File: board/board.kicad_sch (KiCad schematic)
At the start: 2 parts, among them J1 011_GPIO

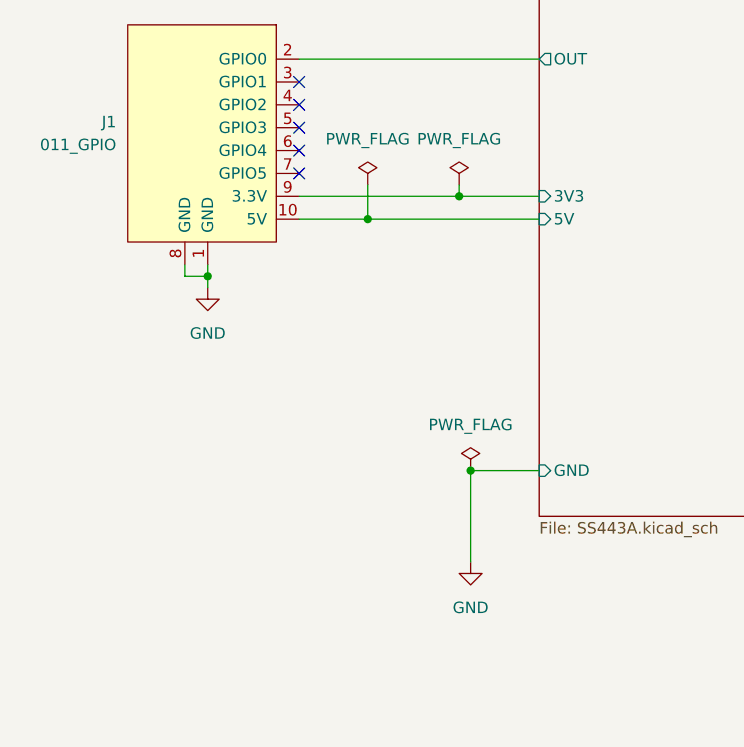
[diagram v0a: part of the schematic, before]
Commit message: Update libraries
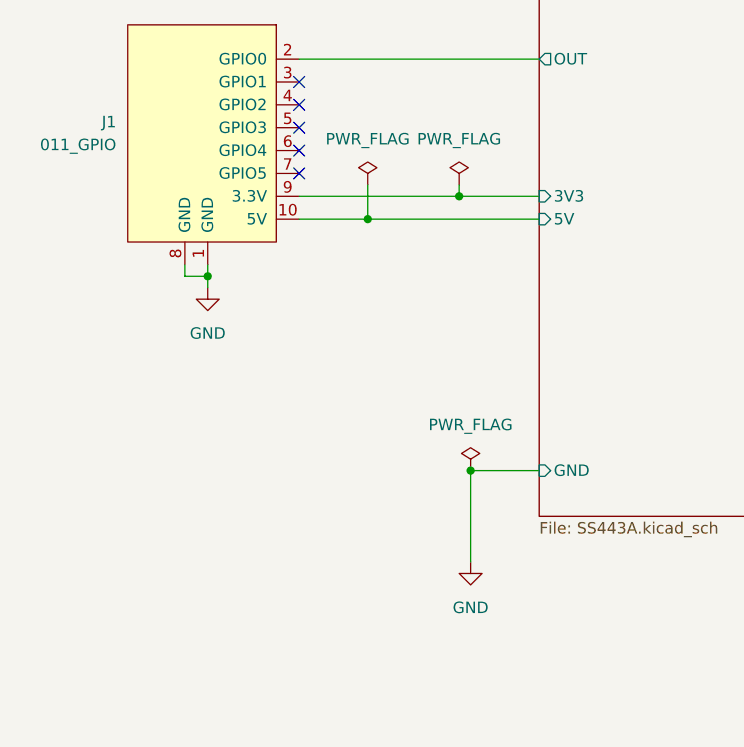
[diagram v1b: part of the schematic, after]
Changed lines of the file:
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@@
   (junction (at 124.46 90.17) (diameter 0) (color 0 0 0 0)
   )
+  (junction (at 96.52 99.06) (diameter 0) (color 0 0 0 0)
+  )
   (junction (at 125.73 120.65) (diameter 0) (color 0 0 0 0)
-  )
-  (junction (at 96.52 99.06) (diameter 0) (color 0 0 0 0)
   )
   (junction (at 114.3 92.71) (diameter 0) (color 0 0 0 0)
@@
     (stroke (width 0) (type default) (color 0 0 0 0))
   )
-  (symbol (lib_id "power:PWR_FLAG") (at 124.46 88.9 0) (mirror y) (unit 1)
-    (in_bom yes) (on_board yes) (fields_autoplaced)
-    (property "Reference" "#FLG0102" (id 0) (at 124.46 86.995 0)
+  (symbol (lib_id "power:PWR_FLAG") (at 124.46 88.9 0) (unit 1)
+    (in_bom yes) (on_board yes) (fields_autoplaced)
+    (property "Reference" "#FLG0103" (id 0) (at 124.46 86.995 0)
       (effects (font (size 1.27 1.27)) hide)
     )
@@
     (pin "1")
   )
-  (symbol (lib_id "power:PWR_FLAG") (at 125.73 120.65 0) (mirror y) (unit 1)
-    (in_bom yes) (on_board yes) (fields_autoplaced)
-    (property "Reference" "#FLG0103" (id 0) (at 125.73 118.745 0)
-      (effects (font (size 1.27 1.27)) hide)
-    )
-    (property "Value" "PWR_FLAG" (id 1) (at 125.73 115.57 0))
-    (property "Footprint" "" (id 2) (at 125.73 120.65 0)
-      (effects (font (size 1.27 1.27)) hide)
-    )
-    (property "Datasheet" "~" (id 3) (at 125.73 120.65 0)
-      (effects (font (size 1.27 1.27)) hide)
-    )
-    (pin "1")
-  )
-  (symbol (lib_id "power:GND") (at 96.52 100.33 0) (mirror y) (unit 1)
-    (in_bom yes) (on_board yes) (fields_autoplaced)
-    (property "Reference" "#PWR0101" (id 0) (at 96.52 106.68 0)
-      (effects (font (size 1.27 1.27)) hide)
-    )
-    (property "Value" "GND" (id 1) (at 96.52 105.41 0))
-    (property "Footprint" "" (id 2) (at 96.52 100.33 0)
-      (effects (font (size 1.27 1.27)) hide)
-    )
-    (property "Datasheet" "" (id 3) (at 96.52 100.33 0)
-      (effects (font (size 1.27 1.27)) hide)
-    )
-    (pin "1")
-  )
-  (symbol (lib_id "power:GND") (at 125.73 130.81 0) (mirror y) (unit 1)
-    (in_bom yes) (on_board yes) (fields_autoplaced)
-    (property "Reference" "#PWR0102" (id 0) (at 125.73 137.16 0)
-      (effects (font (size 1.27 1.27)) hide)
-    )
-    (property "Value" "GND" (id 1) (at 125.73 135.89 0))
-    (property "Footprint" "" (id 2) (at 125.73 130.81 0)
-      (effects (font (size 1.27 1.27)) hide)
-    )
-    (property "Datasheet" "" (id 3) (at 125.73 130.81 0)
-      (effects (font (size 1.27 1.27)) hide)
-    )
-    (pin "1")
-  )
   (symbol (lib_id "Graphic:Logo_Open_Hardware_Small") (at 273.05 157.48 0) (unit 1)
     (in_bom yes) (on_board yes) (fields_autoplaced)
@@
       (effects (font (size 1.27 1.27)) hide)
     )
-  )
-  (symbol (lib_id "power:PWR_FLAG") (at 114.3 88.9 0) (mirror y) (unit 1)
-    (in_bom yes) (on_board yes) (fields_autoplaced)
-    (property "Reference" "#FLG0101" (id 0) (at 114.3 86.995 0)
-      (effects (font (size 1.27 1.27)) hide)
-    )
-    (property "Value" "PWR_FLAG" (id 1) (at 114.3 83.82 0))
-    (property "Footprint" "" (id 2) (at 114.3 88.9 0)
-      (effects (font (size 1.27 1.27)) hide)
-    )
-    (property "Datasheet" "~" (id 3) (at 114.3 88.9 0)
-      (effects (font (size 1.27 1.27)) hide)
-    )
-    (pin "1")
   )
   (symbol (lib_id "put_on_edge:011_GPIO") (at 95.25 83.82 0) (mirror y) (unit 1)
@@
     (pin "9")
   )
+  (symbol (lib_id "power:GND") (at 96.52 100.33 0) (unit 1)
+    (in_bom yes) (on_board yes) (fields_autoplaced)
+    (property "Reference" "#PWR0102" (id 0) (at 96.52 106.68 0)
+      (effects (font (size 1.27 1.27)) hide)
+    )
+    (property "Value" "GND" (id 1) (at 96.52 105.41 0))
+    (property "Footprint" "" (id 2) (at 96.52 100.33 0)
+      (effects (font (size 1.27 1.27)) hide)
+    )
+    (property "Datasheet" "" (id 3) (at 96.52 100.33 0)
+      (effects (font (size 1.27 1.27)) hide)
+    )
+    (pin "1")
+  )
+  (symbol (lib_id "power:PWR_FLAG") (at 125.73 120.65 0) (unit 1)
+    (in_bom yes) (on_board yes) (fields_autoplaced)
+    (property "Reference" "#FLG0101" (id 0) (at 125.73 118.745 0)
+      (effects (font (size 1.27 1.27)) hide)
+    )
+    (property "Value" "PWR_FLAG" (id 1) (at 125.73 115.57 0))
+    (property "Footprint" "" (id 2) (at 125.73 120.65 0)
+      (effects (font (size 1.27 1.27)) hide)
+    )
+    (property "Datasheet" "~" (id 3) (at 125.73 120.65 0)
+      (effects (font (size 1.27 1.27)) hide)
+    )
+    (pin "1")
+  )
+  (symbol (lib_id "power:PWR_FLAG") (at 114.3 88.9 0) (unit 1)
+    (in_bom yes) (on_board yes) (fields_autoplaced)
+    (property "Reference" "#FLG0102" (id 0) (at 114.3 86.995 0)
+      (effects (font (size 1.27 1.27)) hide)
+    )
+    (property "Value" "PWR_FLAG" (id 1) (at 114.3 83.82 0))
+    (property "Footprint" "" (id 2) (at 114.3 88.9 0)
+      (effects (font (size 1.27 1.27)) hide)
+    )
+    (property "Datasheet" "~" (id 3) (at 114.3 88.9 0)
+      (effects (font (size 1.27 1.27)) hide)
+    )
+    (pin "1")
+  )
+  (symbol (lib_id "power:GND") (at 125.73 130.81 0) (unit 1)
+    (in_bom yes) (on_board yes) (fields_autoplaced)
+    (property "Reference" "#PWR0101" (id 0) (at 125.73 137.16 0)
+      (effects (font (size 1.27 1.27)) hide)
+    )
+    (property "Value" "GND" (id 1) (at 125.73 135.89 0))
+    (property "Footprint" "" (id 2) (at 125.73 130.81 0)
+      (effects (font (size 1.27 1.27)) hide)
+    )
+    (property "Datasheet" "" (id 3) (at 125.73 130.81 0)
+      (effects (font (size 1.27 1.27)) hide)
+    )
+    (pin "1")
+  )
   (sheet (at 133.35 63.5) (size 60.96 62.23) (fields_autoplaced)
     (stroke (width 0.1524) (type solid) (color 0 0 0 0))
@@
   )
   (symbol_instances
-    (path "/c62ad806-fea5-41ef-a755-e66e827484f9"
+    (path "/f2d06fe3-e17a-439f-987f-233cdbb94a17"
       (reference "#FLG0101") (unit 1) (value "PWR_FLAG") (footprint "")
     )
-    (path "/124142d5-bbce-45f1-aff2-4ee2b1b91912"
+    (path "/f34909f4-c0ae-4446-a26e-233b5f8a3def"
       (reference "#FLG0102") (unit 1) (value "PWR_FLAG") (footprint "")
     )
-    (path "/2260939c-595d-4925-b584-9d026f14f305"
+    (path "/567f7cbb-a905-4814-8877-d83c2b190d90"
       (reference "#FLG0103") (unit 1) (value "PWR_FLAG") (footprint "")
     )
-    (path "/26138e49-f496-49f7-932c-bede23666c2b"
+    (path "/f6a95196-8c16-41ec-bbc8-c10bf185f315"
       (reference "#PWR0101") (unit 1) (value "GND") (footprint "")
     )
-    (path "/5b5232a0-86b8-4be6-bc95-953eac178a5c"
+    (path "/e271bef5-15e4-40c9-876c-89aee48ff184"
       (reference "#PWR0102") (unit 1) (value "GND") (footprint "")
     )
